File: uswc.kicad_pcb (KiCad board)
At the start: 2 copper layers, 29.3 x 26.8 mm, 48 parts, among them J1 USB_C_Receptacle_USB2.0_16P, J2 Conn_01x02_Socket, P1 DFP, U1 ADG884xRM, U10 SRV05-4, U2 W25Q32JVZP, U3 SN74LVC1T45DBV, U4 RP2040, U5 XC6206PxxxMR, U6 74LVC1G125, U7 CH334F, U8 ADG884xRM, U9 SRV05-4, Y2 12MHz 10ppm

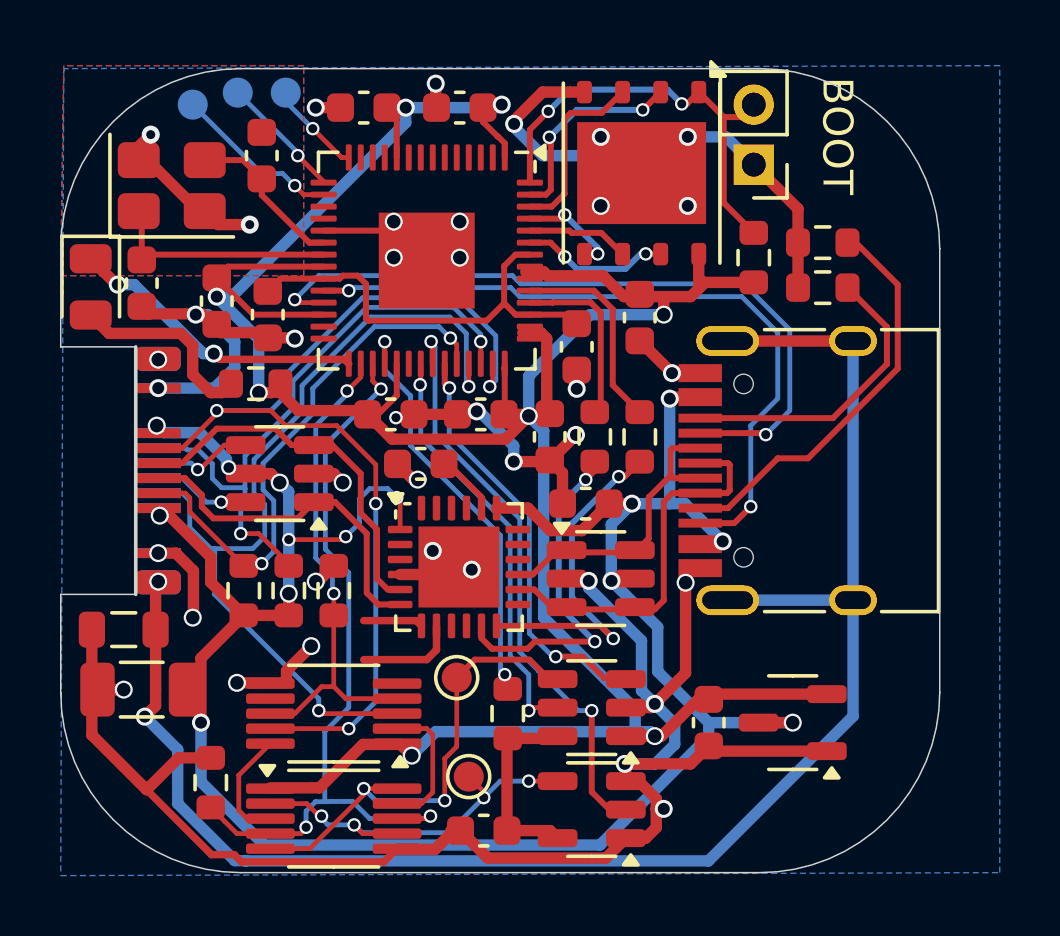
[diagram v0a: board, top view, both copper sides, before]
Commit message: v0.4
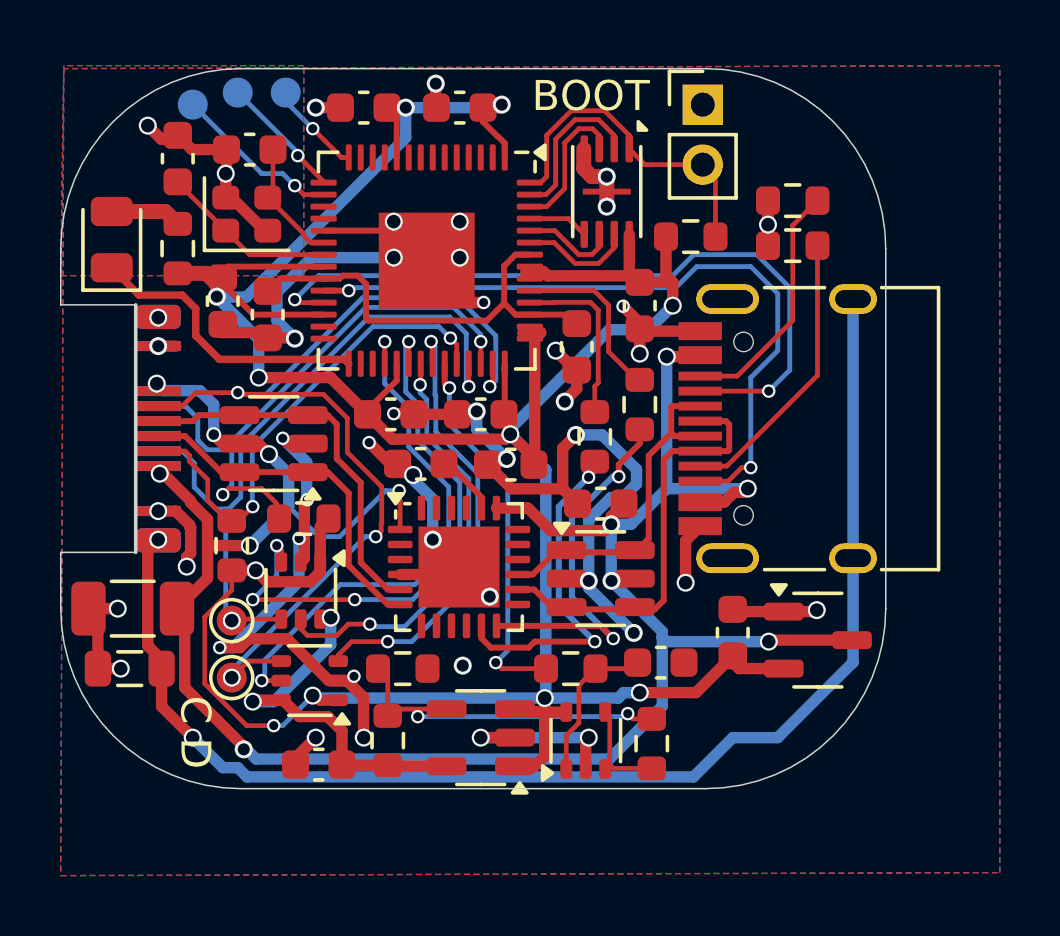
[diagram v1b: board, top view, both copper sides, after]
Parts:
- added C5: 0.1u, Capacitor_SMD:C_0603_1608Metric, F.Cu at (62.1, 127.2)
- added R10: 118k, Resistor_SMD:R_0603_1608Metric, F.Cu at (73.2, 126.5)
- C2: value 10u -> 0.1u
- R5: value 56k -> 10k
- R6: value 56k -> 64.9k
- R8, R9: value 56k -> 36k
- TP1: value SWC_L -> SBU_D
- TP2: value SWD_L -> SBU_C
- U1: value ADG884xRM -> LMV321; footprint Package_SO:MSOP-10_3x3mm_P0.5mm -> Package_TO_SOT_SMD:SOT-353_SC-70-5
- U2: footprint Package_SON:WSON-8-1EP_6x5mm_P1.27mm_EP3.4x4.3mm -> Package_SON:Winbond_USON-8-1EP_3x2mm_P0.5mm_EP0.2x1.6mm
- U3: footprint Package_TO_SOT_SMD:SOT-23-6 -> Package_TO_SOT_SMD:SOT-363_SC-70-6
- U6: value 74LVC1G125 -> SN74LVC1T45DBV; footprint Package_TO_SOT_SMD:SOT-23-5 -> Package_TO_SOT_SMD:SOT-363_SC-70-6
- U8: value ADG884xRM -> MCP1824; footprint Package_SO:MSOP-10_3x3mm_P0.5mm -> Package_TO_SOT_SMD:TSOT-23-5
- Y2: footprint Crystal:Crystal_SMD_3225-4Pin_3.2x2.5mm -> Crystal:Crystal_SMD_2016-4Pin_2.0x1.6mm
- moved U6 12.1 mm to (61.5, 121.4), turned to -90 degrees
- moved U3 9.44 mm to (61.8, 124.4)
- moved TP1 8.56 mm to (59.2, 124.3)
- moved U1 8.45 mm to (71.0, 126.4), turned to 90 degrees
- moved C2 8.13 mm to (73.5, 123.8), turned to 0 degrees
- moved TP2 7.74 mm to (59.2, 122.4)
- moved R6 6.06 mm to (64.4, 126.4), turned to 90 degrees
- moved U8 5.59 mm to (67.5, 126.3), turned to 180 degrees
- moved R15 5.20 mm to (57.4, 110.0), turned to -90 degrees
- moved C17 4.32 mm to (57.4, 107.0), turned to 90 degrees
- moved R5 3.47 mm to (64.9, 124.0), turned to 0 degrees
- moved C19 3.10 mm to (75.9, 122.8), turned to 90 degrees
- moved R2 3.07 mm to (77.9, 108.4)
- moved U5 2.87 mm to (78.7, 123.0), turned to 0 degrees
- moved C15 2.72 mm to (55.9, 122.0)
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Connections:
- C2 pad 1: DUT_VREF -> Net-(U1-+)
- P1 pad A8: DUT_SBU_A -> SBU_D
- P1 pad B6: AUX_D+ -> unconnected-(P1-D+-PadB6)
- P1 pad B7: AUX_D- -> unconnected-(P1-D--PadB7)
- P1 pad B8: DUT_SBU_B -> SBU_C
- R5 pad 1: GND -> Net-(U8-SENSE/ADJ)
- R5 pad 2: DUT_SWD_CONN -> GND
- R6 pad 1: GND -> DUT_VREF
- R6 pad 2: DUT_SWD_SWAP -> Net-(U8-SENSE/ADJ)
- R7 pad 1: DUT_VREF -> Net-(U1-+)
- R8 pad 2: VBUS -> +3V3
- R9 pad 2: VBUS -> +3V3
- TP1 pad 1: DUT_SWC_L -> SBU_D
- TP2 pad 1: DUT_SWD_L -> SBU_C
- U1 pad 1: +3V3 -> Net-(U1-+)
- U1 pad 2: DUT_SWC/D_SBU -> GND
- U1 pad 3: DUT_SBU_B -> MARGIN
- U1 pad 4: DUT_SWD_CONN -> MARGIN
- U1 pad 5: unconnected-(U1-S1B-Pad5) -> +3V3
- U10 pad 4: AUX_D+ -> DUT_D-
- U10 pad 6: AUX_D- -> DUT_D+
- U3 pad 4: DUT_SWD_L -> SBU_D
- U3 pad 5: DUT_SWDIR -> DUT_SWDIR_D
- U4 pad 30: DUT_SWD_CONN -> unconnected-(U4-GPIO19-Pad30)
- U4 pad 31: DUT_SWD_SWAP -> unconnected-(U4-GPIO20-Pad31)
- U4 pad 32: PWM -> DUT_SWDIR_D
- U4 pad 34: unconnected-(U4-GPIO22-Pad34) -> DUT_SWC
- U4 pad 35: DUT_SWDIR -> DUT_SWDIR_C
- U4 pad 36: DUT_SWC -> DUT_SWD
- U4 pad 37: DUT_SWD -> PWM
- U4 pad 39: DUT_SBU_B -> SBU_C
- U4 pad 41: DUT_SBU_A -> SBU_D
- U6 pad 1: GND -> +3V3
- U6 pad 2: DUT_SWC -> GND
- U6 pad 3: GND -> DUT_SWC
- U6 pad 4: DUT_SWC_L -> SBU_C
- U6 pad 5: DUT_VREF -> DUT_SWDIR_C
- U8 pad 2: DUT_SWC_L -> GND
- U8 pad 3: DUT_SWD/C_SBU -> +3V3
- U8 pad 4: DUT_SWD_SWAP -> Net-(U8-SENSE/ADJ)
- U8 pad 5: DUT_SWD_L -> DUT_VREF
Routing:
- net DUT_SBU_A: track 34.7 -> 0.00 mm, vias 4 -> 0
- net SBU_D: track 0.00 -> 32.9 mm, vias 0 -> 4
- net DUT_SBU_B: track 29.6 -> 0.00 mm, vias 2 -> 0
- net DUT_SWD_SWAP: track 26.0 -> 0.00 mm, vias 3 -> 0
- net SBU_C: track 0.00 -> 23.5 mm, vias 0 -> 2
- net DUT_SWDIR_D: track 0.00 -> 17.6 mm, vias 0 -> 2
- net DUT_SWD_L: track 16.6 -> 0.00 mm, vias 2 -> 0
- net DUT_SWD_CONN: track 16.4 -> 0.00 mm, vias 2 -> 0
- net +3V3: track 99.0 -> 114.6 mm, vias 8 -> 11
- net GND: track 113.3 -> 98.2 mm, vias 37 -> 44
- net DUT_SWDIR_C: track 0.00 -> 14.4 mm, vias 0 -> 2
- net DUT_SWDIR: track 14.1 -> 0.00 mm, vias 2 -> 0
- net DUT_SWC_L: track 13.5 -> 0.00 mm, vias 4 -> 0
- net Net-(U8-SENSE/ADJ): track 0.00 -> 11.7 mm, vias 0 -> 2
- net SHIELD: track 54.2 -> 43.6 mm
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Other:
- board size 29.3 x 26.8 mm -> 27.5 x 24 mm
- board text added: "C D"
- board text added: "v0.4"
- board text removed: "JLCJLCJLCJLC"
- board text removed: "v0.3"
